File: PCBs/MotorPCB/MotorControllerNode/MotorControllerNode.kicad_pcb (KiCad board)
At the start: 4 copper layers, 100 x 100 mm, 32 parts, among them IC1 DAC53202RTER, IC2 TXS0108EQPWRQ1, IC3 TXS0108EQPWRQ1, J2 DSUB9 J1, J3 Encoder, J4 GPIO, J5 DSUB9 to backplane, J6 Battery negative, J7 Reversing contactor 1, J8 Reversing contactor 2, J9 DSUB15 J2, Q1 NPN, U1 ESP32-S3-DevKitC, U2 SN65HVD230, U3 J104D2C5VDC.20S

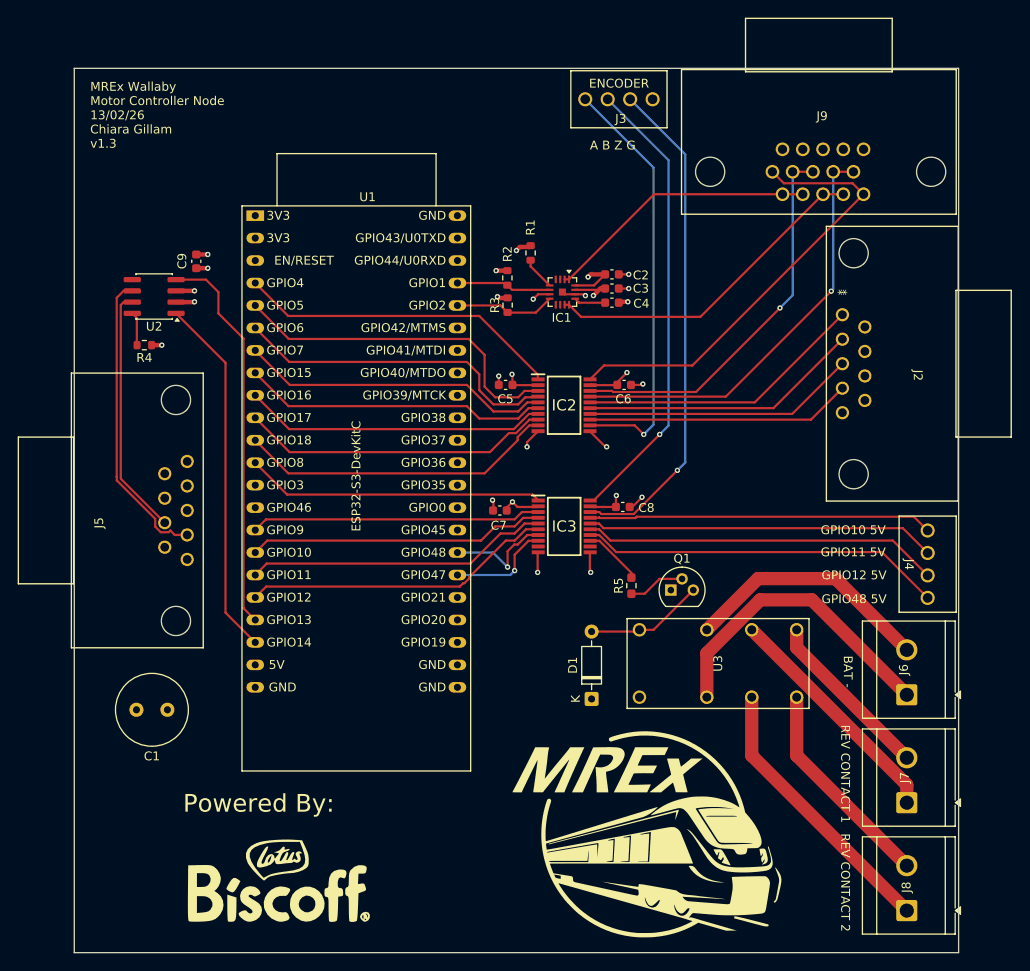
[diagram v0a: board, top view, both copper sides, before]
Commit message: Revert "added driver controls v2"
This reverts commit c73e8f860f70517a898f0b3e351800c05ab551df.
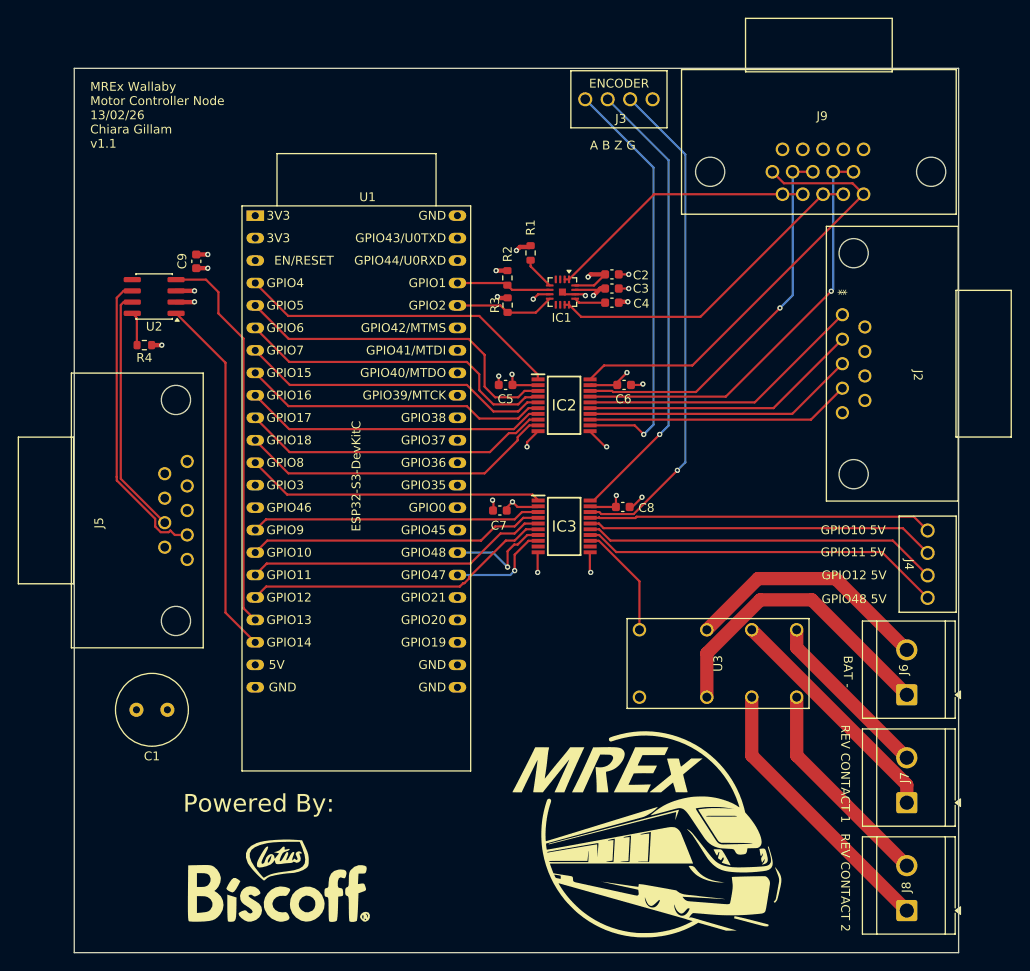
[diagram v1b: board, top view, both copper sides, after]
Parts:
- removed D1: 1N914, Diode_THT:D_DO-35_SOD27_P7.62mm_Horizontal
- removed Q1: NPN, Package_TO_SOT_THT:TO-92
- removed R5: 1k, Resistor_SMD:R_0603_1608Metric_Pad0.98x0.95mm_HandSolder
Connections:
- U3 pad 8: Net-(D1-A) -> /GPIO47 Reversing Contactor
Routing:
- net Net-(D1-A): track 13.0 -> 0.00 mm
- net Net-(Q1-B): track 6.43 -> 0.00 mm
- net /GPIO47 Reversing Contactor: track 6.70 -> 13.0 mm
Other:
- board text added: "MREx Wallaby Motor Controller Node 13/02/26 Chiara Gillam v1.1"
- board text removed: "MREx Wallaby Motor Controller Node 13/02/26 Chiara Gillam v1.3"

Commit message: Reapply "added driver controls v2"
This reverts commit d70487c3c1110107dce6cdfc2b36a156bfb5c696.
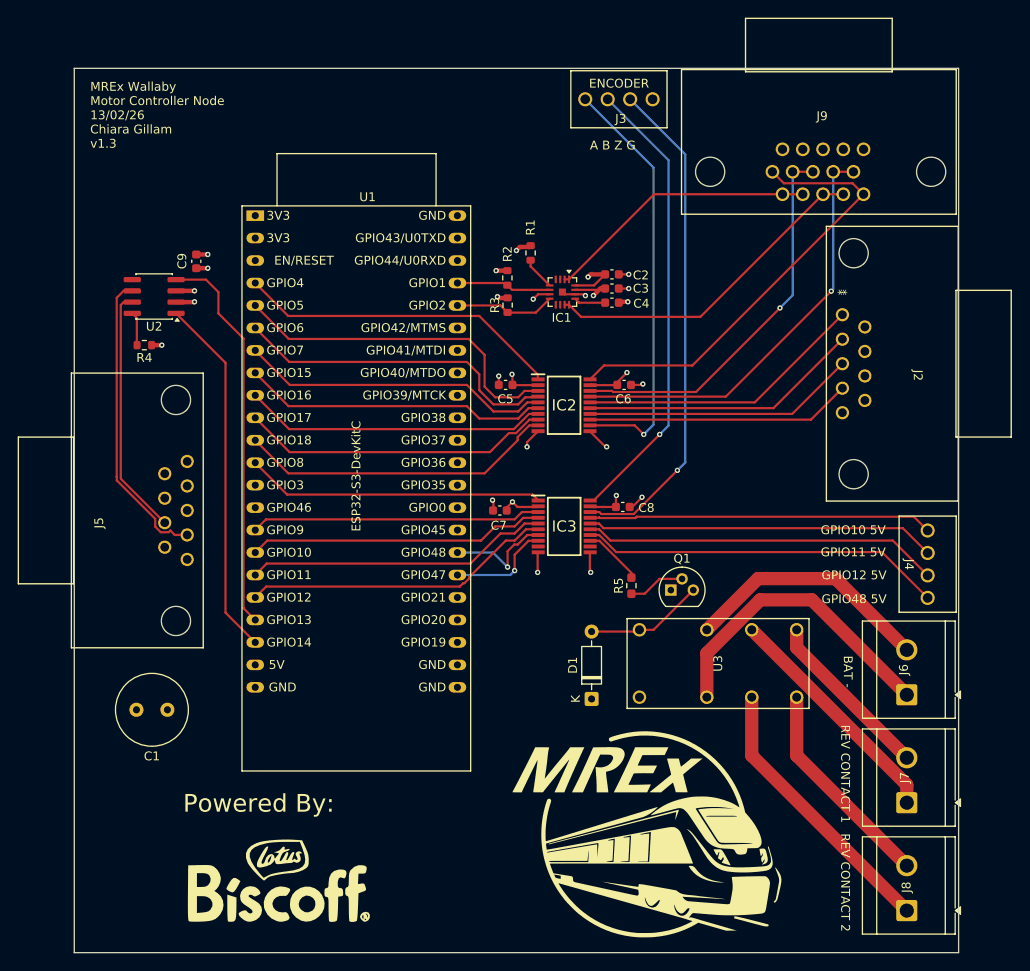
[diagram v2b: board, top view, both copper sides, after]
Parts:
- added D1: 1N914, Diode_THT:D_DO-35_SOD27_P7.62mm_Horizontal, F.Cu at (83.5, 96.3)
- added Q1: NPN, Package_TO_SOT_THT:TO-92, F.Cu at (92.5, 84.0)
- added R5: 1k, Resistor_SMD:R_0603_1608Metric_Pad0.98x0.95mm_HandSolder, F.Cu at (88.0, 83.5)
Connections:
- U3 pad 8: /GPIO47 Reversing Contactor -> Net-(D1-A)
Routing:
- net Net-(D1-A): track 0.00 -> 13.0 mm
- net Net-(Q1-B): track 0.00 -> 6.43 mm
- net /GPIO47 Reversing Contactor: track 13.0 -> 6.70 mm
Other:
- board text added: "MREx Wallaby Motor Controller Node 13/02/26 Chiara Gillam v1.3"
- board text removed: "MREx Wallaby Motor Controller Node 13/02/26 Chiara Gillam v1.1"
